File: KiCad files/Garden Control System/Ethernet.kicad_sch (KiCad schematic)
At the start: 26 parts, among them J1 RJHSE-5084, T1 HX1188FNL, U2 DP83826IRHBR, Y2 ECS-250-20-33-TR

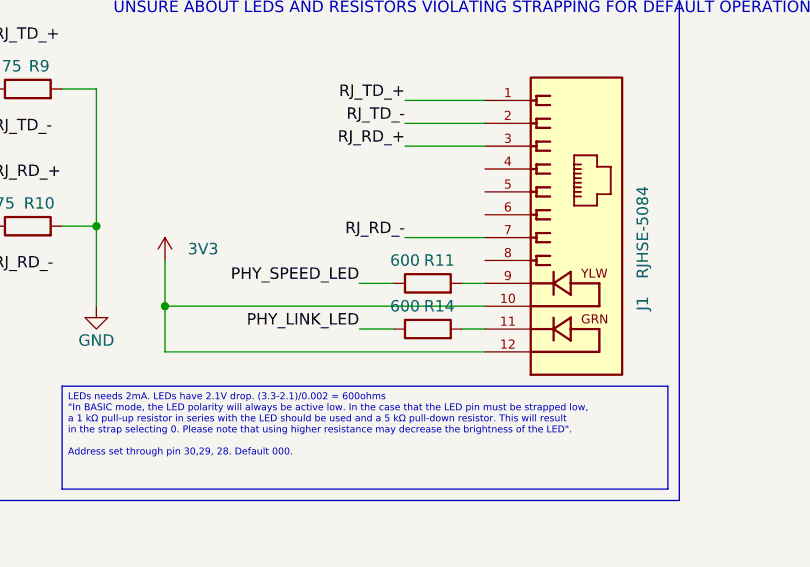
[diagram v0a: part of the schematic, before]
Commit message: working on temp sensor circuit
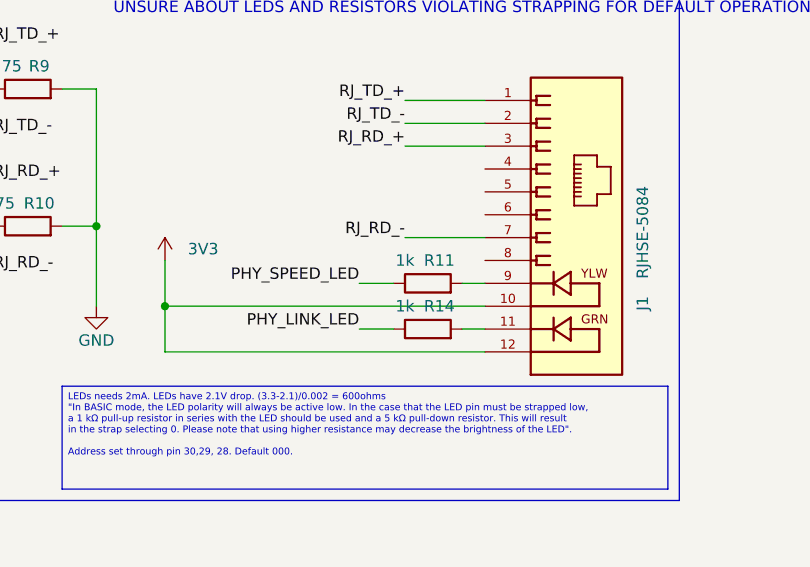
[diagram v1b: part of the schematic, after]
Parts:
- R11, R14: value 600 -> 1k
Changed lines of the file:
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@@
 			)
 		)
-		(property "Value" "600"
+		(property "Value" "1k"
 			(at 254 46.99 90)
 			(effects
@@
 			)
 		)
-		(property "Value" "600"
+		(property "Value" "1k"
 			(at 254 52.07 90)
 			(effects

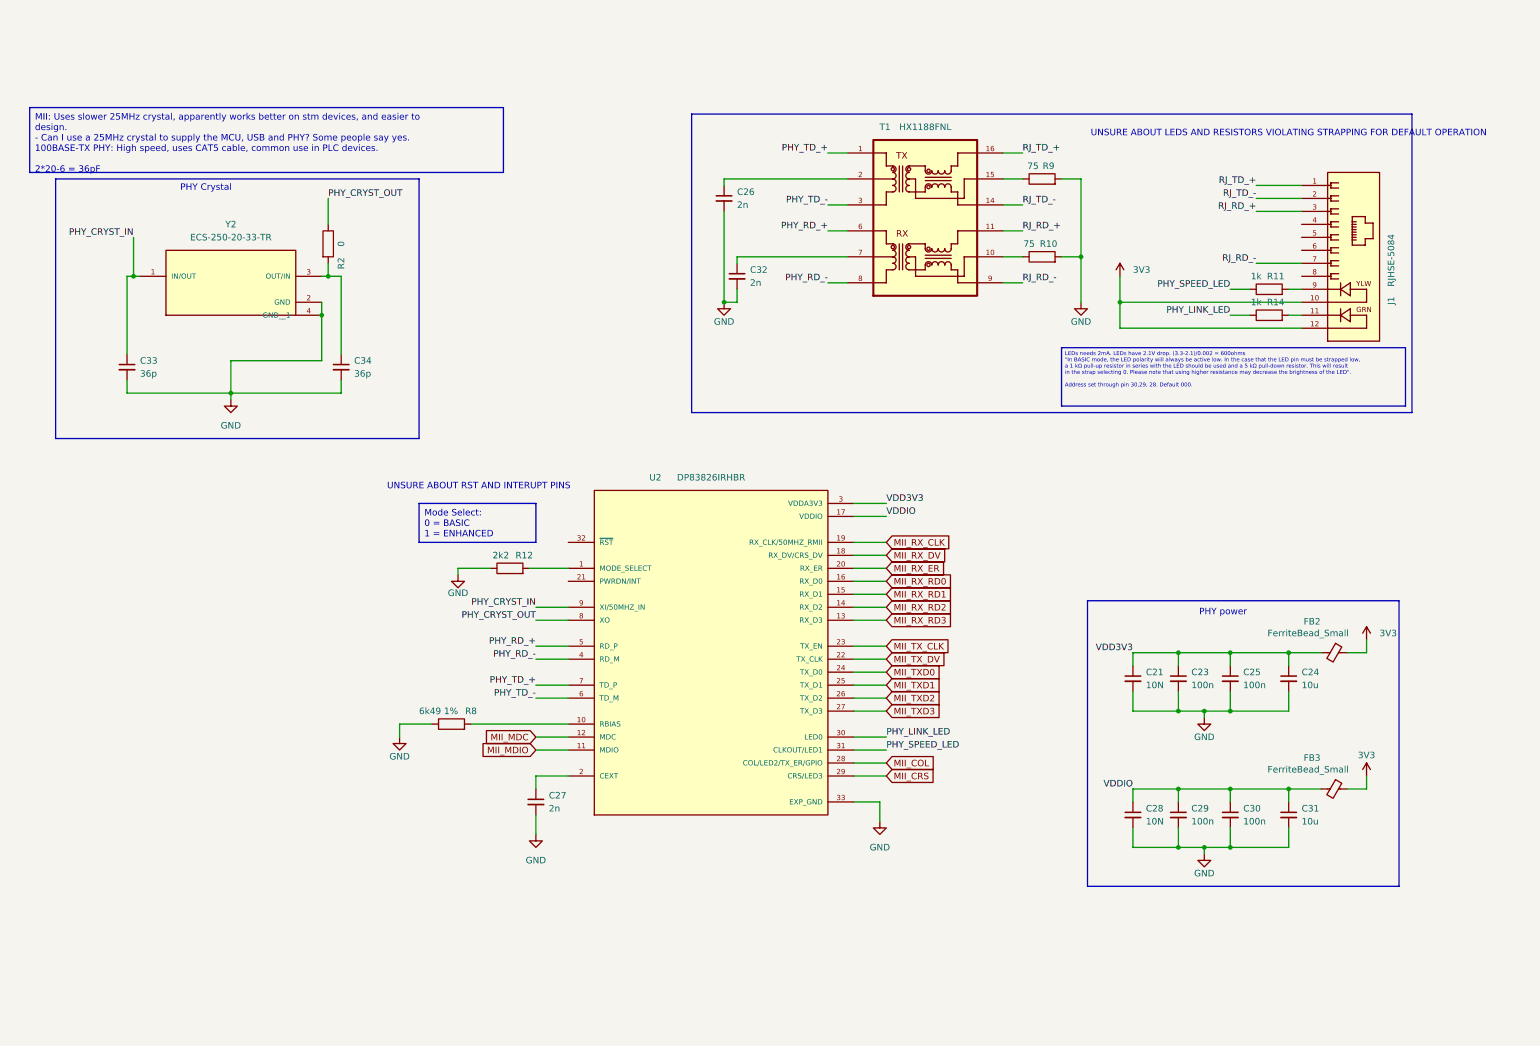
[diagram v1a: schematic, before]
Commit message: we cookin' again. Added LSD and start temp sense section.
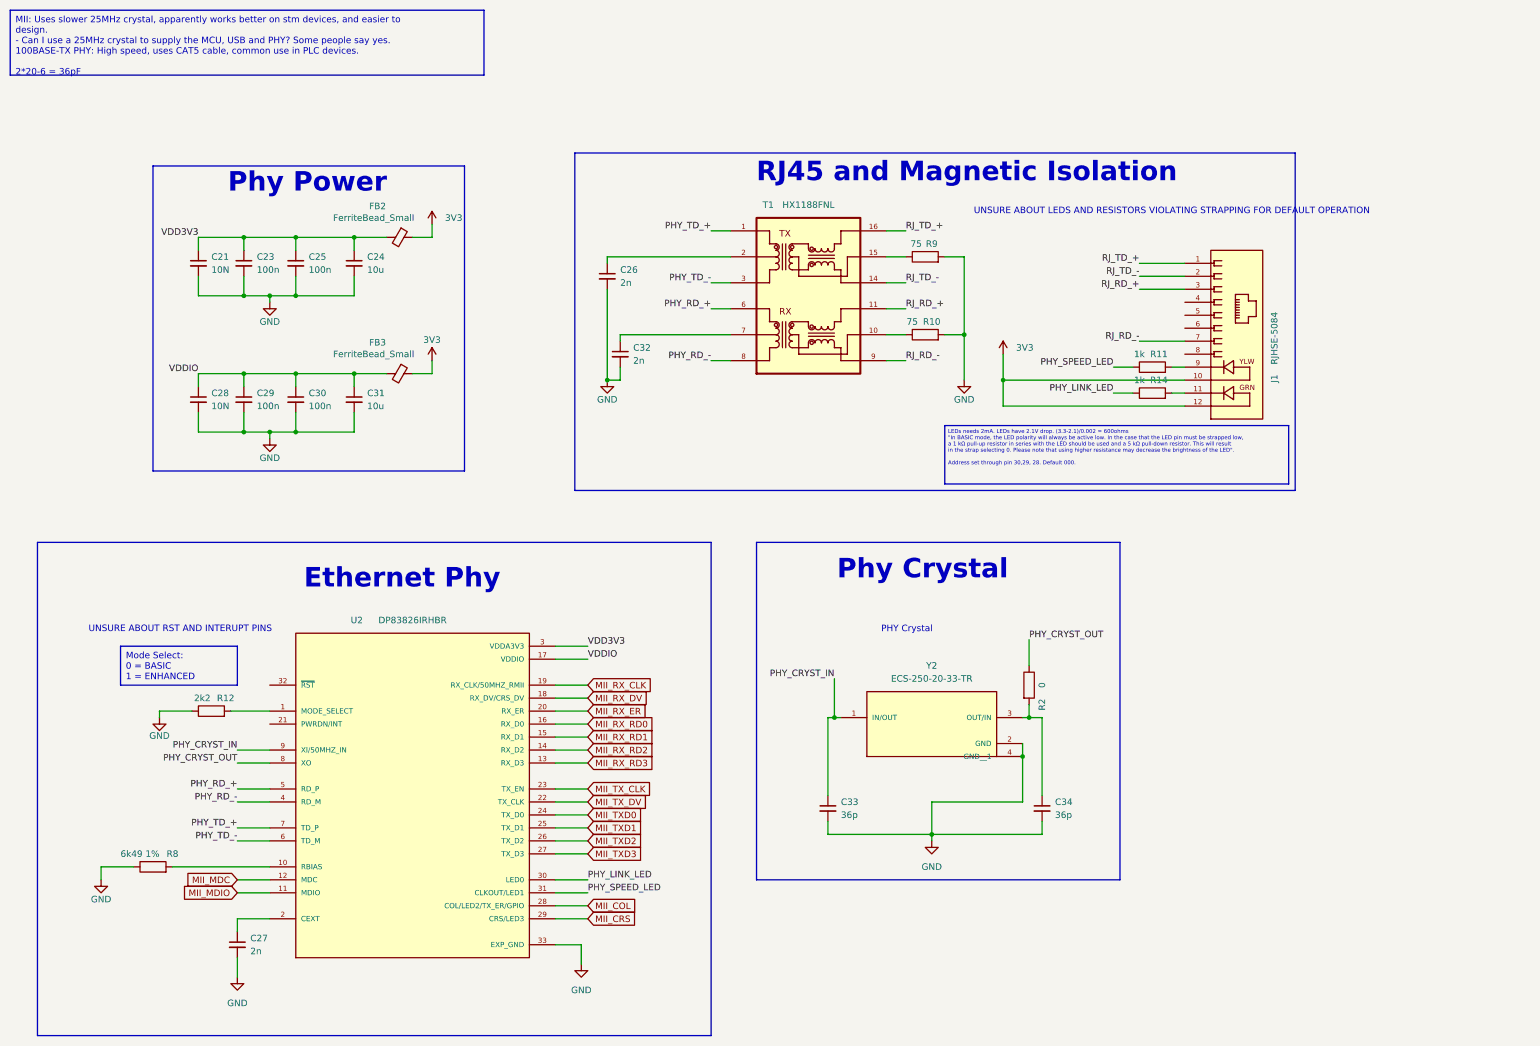
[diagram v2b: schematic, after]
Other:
- note added: "Ethernet Phy"
- note added: "Phy Crystal"
- note added: "Phy Power"
- note added: "RJ45 and Magnetic Isolation"
- note removed: "PHY power"
- moved on the sheet: C21, C23, C24, C25, C26, C27, C28, C29, C30, C31, C32, C33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
